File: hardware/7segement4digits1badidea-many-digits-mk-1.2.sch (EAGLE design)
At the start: 8 parts

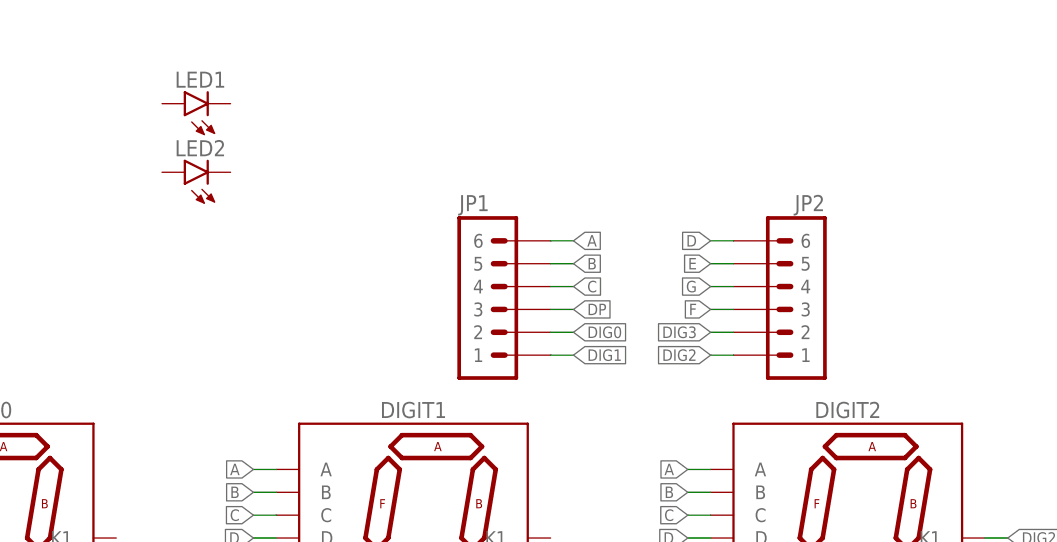
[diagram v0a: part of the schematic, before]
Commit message: lots of terribad ideas here
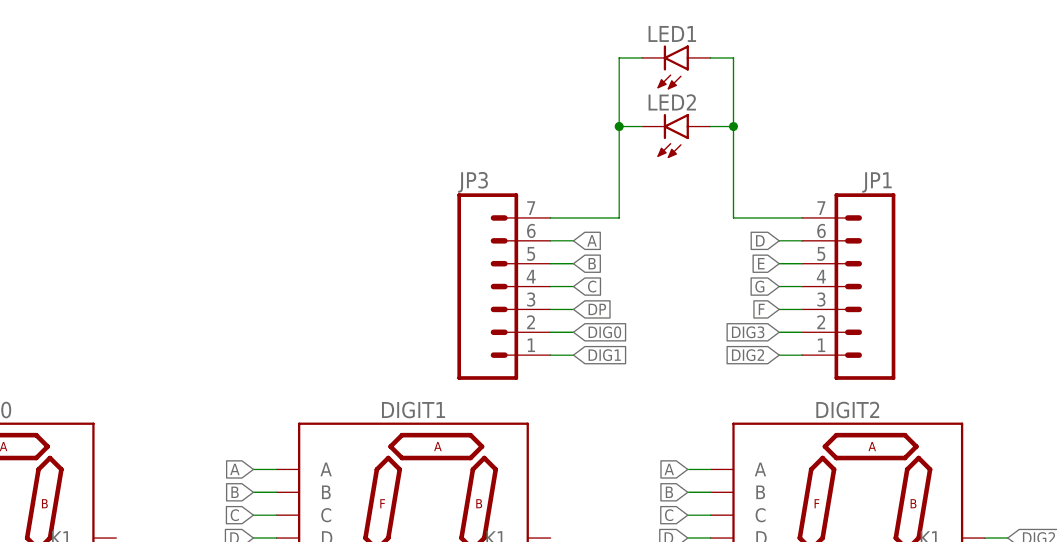
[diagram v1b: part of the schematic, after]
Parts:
- removed JP2: M06-NOBS-PTH, A_butts:M06-NOBS-PTH
- added JP3: (no value), A_butts:M07
- JP1: value M06-NOBS-PTH -> (none); device A_butts:M06-NOBS-PTH -> A_butts:M07
- LED1, LED2: value LED3MM -> LED3MM-LESS; device A_butts:LED3MM -> A_butts:LED3MM-LESS
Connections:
- new net N$2: JP3.7, LED1.C, LED2.C
- new net N$3: JP1.7, LED1.A, LED2.A
- net A: now also JP3.6; no longer JP1.6
- net B: now also JP3.5; no longer JP1.5
- net C: now also JP3.4; no longer JP1.4
- net D: now also JP1.6; no longer JP2.6
- net DIG0: now also JP3.2; no longer JP1.2
- net DIG1: now also JP3.1; no longer JP1.1
- net DIG2: now also JP1.1; no longer JP2.1
- net DIG3: now also JP1.2; no longer JP2.2
- net DP: now also JP3.3; no longer JP1.3
- net E: now also JP1.5; no longer JP2.5
- net F: now also JP1.3; no longer JP2.3
- net G: now also JP1.4; no longer JP2.4
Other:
- moved on the sheet: LED1, LED2
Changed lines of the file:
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@@
 <setting verticaltext="up"/>
 </settings>
-<grid distance="100" unitdist="mil" unit="mil" style="lines" multiple="1" display="yes" altdistance="1" altunitdist="mil" altunit="mil"/>
+<grid distance="100" unitdist="mil" unit="mil" style="lines" multiple="1" display="yes" altdistance="2" altunitdist="mil" altunit="mil"/>
 <layers>
 <layer number="1" name="Top" color="4" fill="1" visible="yes" active="no"/>
@@
 <part name="DIGIT2" library="A_butts" deviceset="7SEG_1DIG" device="PTH-10MM"/>
 <part name="DIGIT3" library="A_butts" deviceset="7SEG_1DIG" device="PTH-10MM"/>
-<part name="JP1" library="A_butts" deviceset="M06" device="-NOBS-PTH"/>
-<part name="JP2" library="A_butts" deviceset="M06" device="-NOBS-PTH"/>
-<part name="LED1" library="A_butts" deviceset="LED" device="3MM"/>
-<part name="LED2" library="A_butts" deviceset="LED" device="3MM"/>
+<part name="LED1" library="A_butts" deviceset="LED" device="3MM-LESS" value="LED3MM-LESS"/>
+<part name="LED2" library="A_butts" deviceset="LED" device="3MM-LESS" value="LED3MM-LESS"/>
+<part name="JP3" library="A_butts" deviceset="M07" device=""/>
+<part name="JP1" library="A_butts" deviceset="M07" device=""/>
 </parts>
 <sheets>
@@
 <instance part="DIGIT2" gate="G$1" x="119.38" y="53.34"/>
 <instance part="DIGIT3" gate="G$1" x="167.64" y="53.34"/>
-<instance part="JP1" gate="G$1" x="81.28" y="81.28"/>
-<instance part="JP2" gate="G$1" x="111.76" y="81.28" rot="MR0"/>
-<instance part="LED1" gate="G$1" x="45.72" y="104.14" rot="R90"/>
-<instance part="LED2" gate="G$1" x="45.72" y="96.52" rot="R90"/>
+<instance part="LED1" gate="G$1" x="101.6" y="109.22" rot="MR90"/>
+<instance part="LED2" gate="G$1" x="101.6" y="101.6" rot="MR90"/>
+<instance part="JP3" gate="G$1" x="81.28" y="81.28"/>
+<instance part="JP1" gate="G$1" x="119.38" y="81.28" rot="MR0"/>
 </instances>
 <busses>
@@
 <wire x1="88.9" y1="88.9" x2="86.36" y2="88.9" width="0.1524" layer="91"/>
 <label x="88.9" y="88.9" size="1.27" layer="95" xref="yes"/>
-<pinref part="JP1" gate="G$1" pin="6"/>
+<pinref part="JP3" gate="G$1" pin="6"/>
 </segment>
 </net>
@@
 <wire x1="88.9" y1="83.82" x2="86.36" y2="83.82" width="0.1524" layer="91"/>
 <label x="88.9" y="83.82" size="1.27" layer="95" xref="yes"/>
-<pinref part="JP1" gate="G$1" pin="4"/>
+<pinref part="JP3" gate="G$1" pin="4"/>
 </segment>
 </net>
@@
 </segment>
 <segment>
-<wire x1="104.14" y1="86.36" x2="106.68" y2="86.36" width="0.1524" layer="91"/>
-<label x="104.14" y="86.36" size="1.27" layer="95" rot="MR0" xref="yes"/>
-<pinref part="JP2" gate="G$1" pin="5"/>
+<wire x1="111.76" y1="86.36" x2="114.3" y2="86.36" width="0.1524" layer="91"/>
+<label x="111.76" y="86.36" size="1.27" layer="95" rot="MR0" xref="yes"/>
+<pinref part="JP1" gate="G$1" pin="5"/>
 </segment>
 </net>
@@
 </segment>
 <segment>
-<wire x1="104.14" y1="83.82" x2="106.68" y2="83.82" width="0.1524" layer="91"/>
-<label x="104.14" y="83.82" size="1.27" layer="95" rot="MR0" xref="yes"/>
-<pinref part="JP2" gate="G$1" pin="4"/>
+<wire x1="111.76" y1="83.82" x2="114.3" y2="83.82" width="0.1524" layer="91"/>
+<label x="111.76" y="83.82" size="1.27" layer="95" rot="MR0" xref="yes"/>
+<pinref part="JP1" gate="G$1" pin="4"/>
 </segment>
 </net>
@@
 <wire x1="88.9" y1="81.28" x2="86.36" y2="81.28" width="0.1524" layer="91"/>
 <label x="88.9" y="81.28" size="1.27" layer="95" rot="MR180" xref="yes"/>
-<pinref part="JP1" gate="G$1" pin="3"/>
+<pinref part="JP3" gate="G$1" pin="3"/>
 </segment>
 </net>
@@
 </segment>
 <segment>
-<wire x1="104.14" y1="88.9" x2="106.68" y2="88.9" width="0.1524" layer="91"/>
-<label x="104.14" y="88.9" size="1.27" layer="95" rot="R180" xref="yes"/>
-<pinref part="JP2" gate="G$1" pin="6"/>
+<wire x1="111.76" y1="88.9" x2="114.3" y2="88.9" width="0.1524" layer="91"/>
+<label x="111.76" y="88.9" size="1.27" layer="95" rot="R180" xref="yes"/>
+<pinref part="JP1" gate="G$1" pin="6"/>
 </segment>
 </net>
@@
 <wire x1="88.9" y1="86.36" x2="86.36" y2="86.36" width="0.1524" layer="91"/>
 <label x="88.9" y="86.36" size="1.27" layer="95" xref="yes"/>
-<pinref part="JP1" gate="G$1" pin="5"/>
+<pinref part="JP3" gate="G$1" pin="5"/>
 </segment>
 </net>
@@
 </segment>
 <segment>
-<wire x1="104.14" y1="81.28" x2="106.68" y2="81.28" width="0.1524" layer="91"/>
-<label x="104.14" y="81.28" size="1.27" layer="95" rot="MR0" xref="yes"/>
-<pinref part="JP2" gate="G$1" pin="3"/>
+<wire x1="111.76" y1="81.28" x2="114.3" y2="81.28" width="0.1524" layer="91"/>
+<label x="111.76" y="81.28" size="1.27" layer="95" rot="MR0" xref="yes"/>
+<pinref part="JP1" gate="G$1" pin="3"/>
 </segment>
 </net>
@@
 <wire x1="86.36" y1="78.74" x2="88.9" y2="78.74" width="0.1524" layer="91"/>
 <label x="88.9" y="78.74" size="1.27" layer="95" xref="yes"/>
-<pinref part="JP1" gate="G$1" pin="2"/>
+<pinref part="JP3" gate="G$1" pin="2"/>
 </segment>
 <segment>
@@
 <wire x1="86.36" y1="76.2" x2="88.9" y2="76.2" width="0.1524" layer="91"/>
 <label x="88.9" y="76.2" size="1.27" layer="95" xref="yes"/>
-<pinref part="JP1" gate="G$1" pin="1"/>
+<pinref part="JP3" gate="G$1" pin="1"/>
 </segment>
 <segment>
@@
 </segment>
 <segment>
-<wire x1="106.68" y1="78.74" x2="104.14" y2="78.74" width="0.1524" layer="91"/>
-<label x="104.14" y="78.74" size="1.27" layer="95" rot="MR0" xref="yes"/>
-<pinref part="JP2" gate="G$1" pin="2"/>
+<wire x1="114.3" y1="78.74" x2="111.76" y2="78.74" width="0.1524" layer="91"/>
+<label x="111.76" y="78.74" size="1.27" layer="95" rot="MR0" xref="yes"/>
+<pinref part="JP1" gate="G$1" pin="2"/>
 </segment>
 </net>
@@
 </segment>
 <segment>
-<wire x1="106.68" y1="76.2" x2="104.14" y2="76.2" width="0.1524" layer="91"/>
-<label x="104.14" y="76.2" size="1.27" layer="95" rot="MR0" xref="yes"/>
-<pinref part="JP2" gate="G$1" pin="1"/>
-</segment>
-</net>
+<wire x1="114.3" y1="76.2" x2="111.76" y2="76.2" width="0.1524" layer="91"/>
+<label x="111.76" y="76.2" size="1.27" layer="95" rot="MR0" xref="yes"/>
+<pinref part="JP1" gate="G$1" pin="1"/>
+</segment>
+</net>
+<net name="N$2" class="0">
+<segment>
+<pinref part="JP3" gate="G$1" pin="7"/>
+<wire x1="86.36" y1="91.44" x2="93.98" y2="91.44" width="0.1524" layer="91"/>
+<wire x1="93.98" y1="91.44" x2="93.98" y2="101.6" width="0.1524" layer="91"/>
+<pinref part="LED2" gate="G$1" pin="C"/>
+<wire x1="93.98" y1="101.6" x2="93.98" y2="109.22" width="0.1524" layer="91"/>
+<wire x1="96.52" y1="101.6" x2="93.98" y2="101.6" width="0.1524" layer="91"/>
+<junction x="93.98" y="101.6"/>
+<pinref part="LED1" gate="G$1" pin="C"/>
+<wire x1="93.98" y1="109.22" x2="96.52" y2="109.22" width="0.1524" layer="91"/>
+</segment>
+</net>
+<net name="N$3" class="0">
+<segment>
+<wire x1="106.68" y1="109.22" x2="106.68" y2="101.6" width="0.1524" layer="91"/>
+<pinref part="JP1" gate="G$1" pin="7"/>
+<wire x1="106.68" y1="101.6" x2="106.68" y2="91.44" width="0.1524" layer="91"/>
+<wire x1="106.68" y1="91.44" x2="114.3" y2="91.44" width="0.1524" layer="91"/>
+<pinref part="LED1" gate="G$1" pin="A"/>
+<wire x1="104.14" y1="109.22" x2="106.68" y2="109.22" width="0.1524" layer="91"/>
+<pinref part="LED2" gate="G$1" pin="A"/>
+<wire x1="104.14" y1="101.6" x2="106.68" y2="101.6" width="0.1524" layer="91"/>
+<junction x="106.68" y="101.6"/>
+</segment>
+</net>
